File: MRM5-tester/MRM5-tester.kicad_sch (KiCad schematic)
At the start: 0 parts

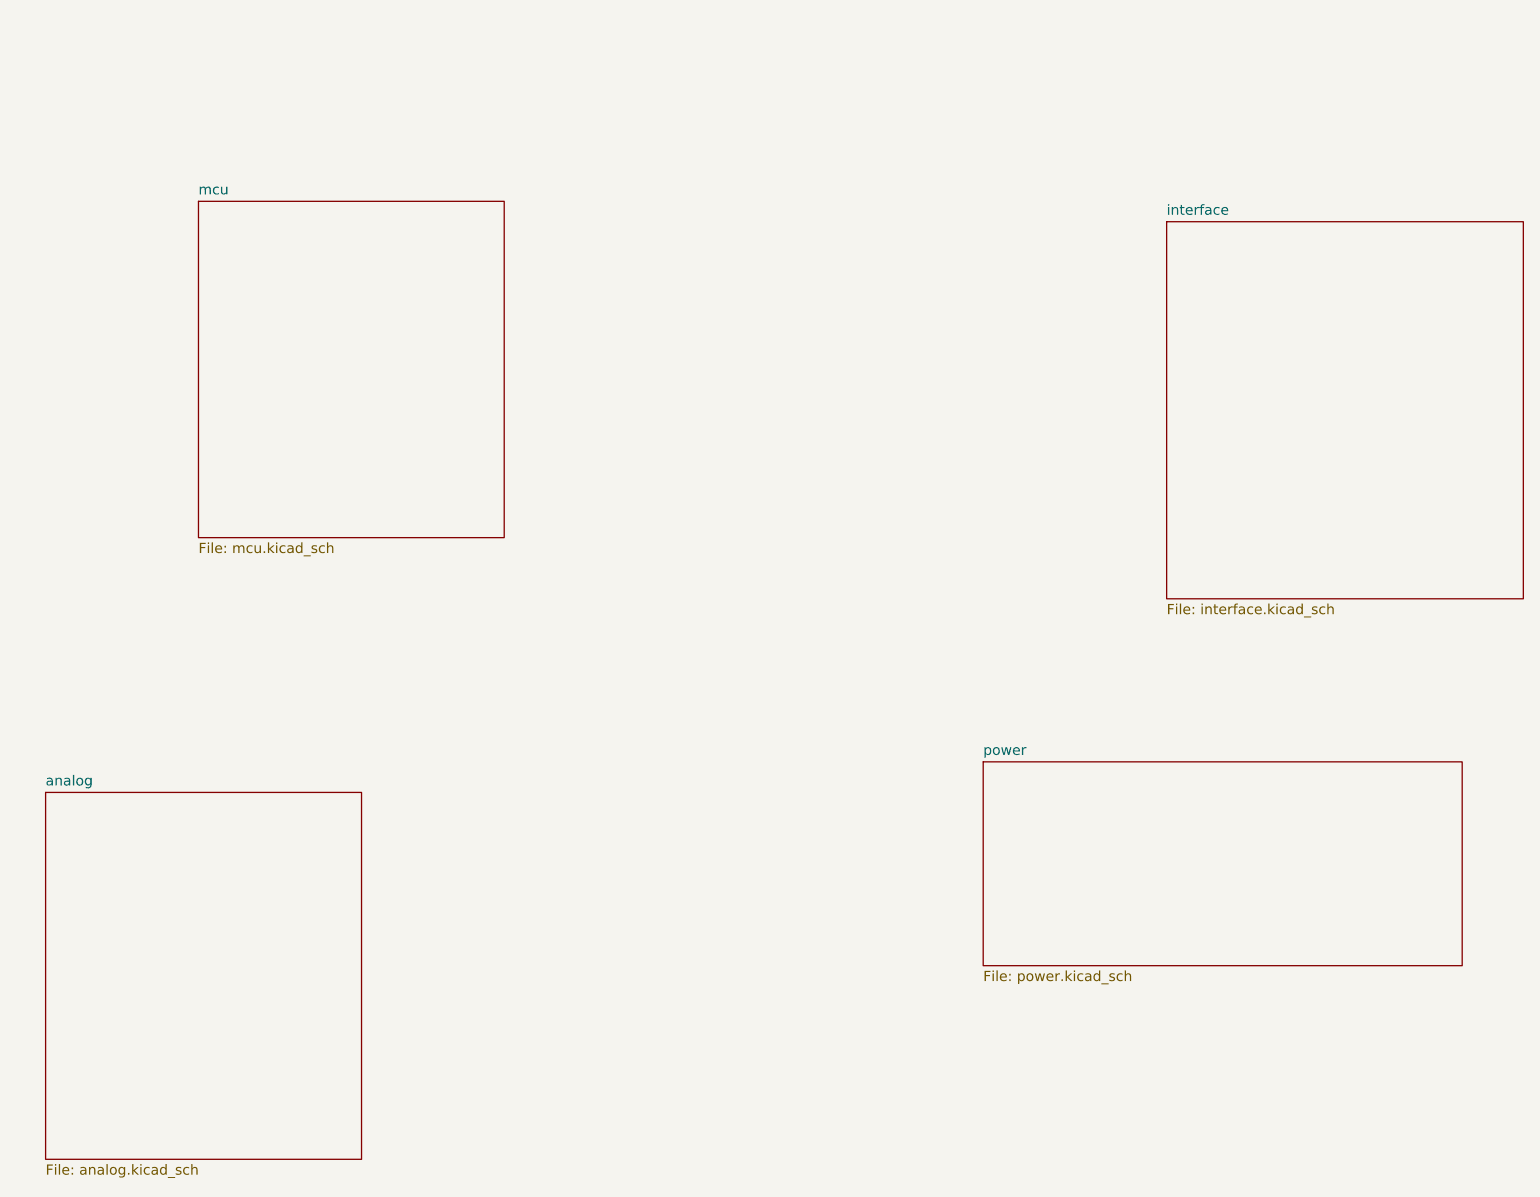
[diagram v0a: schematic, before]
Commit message: tester PCB 작성중
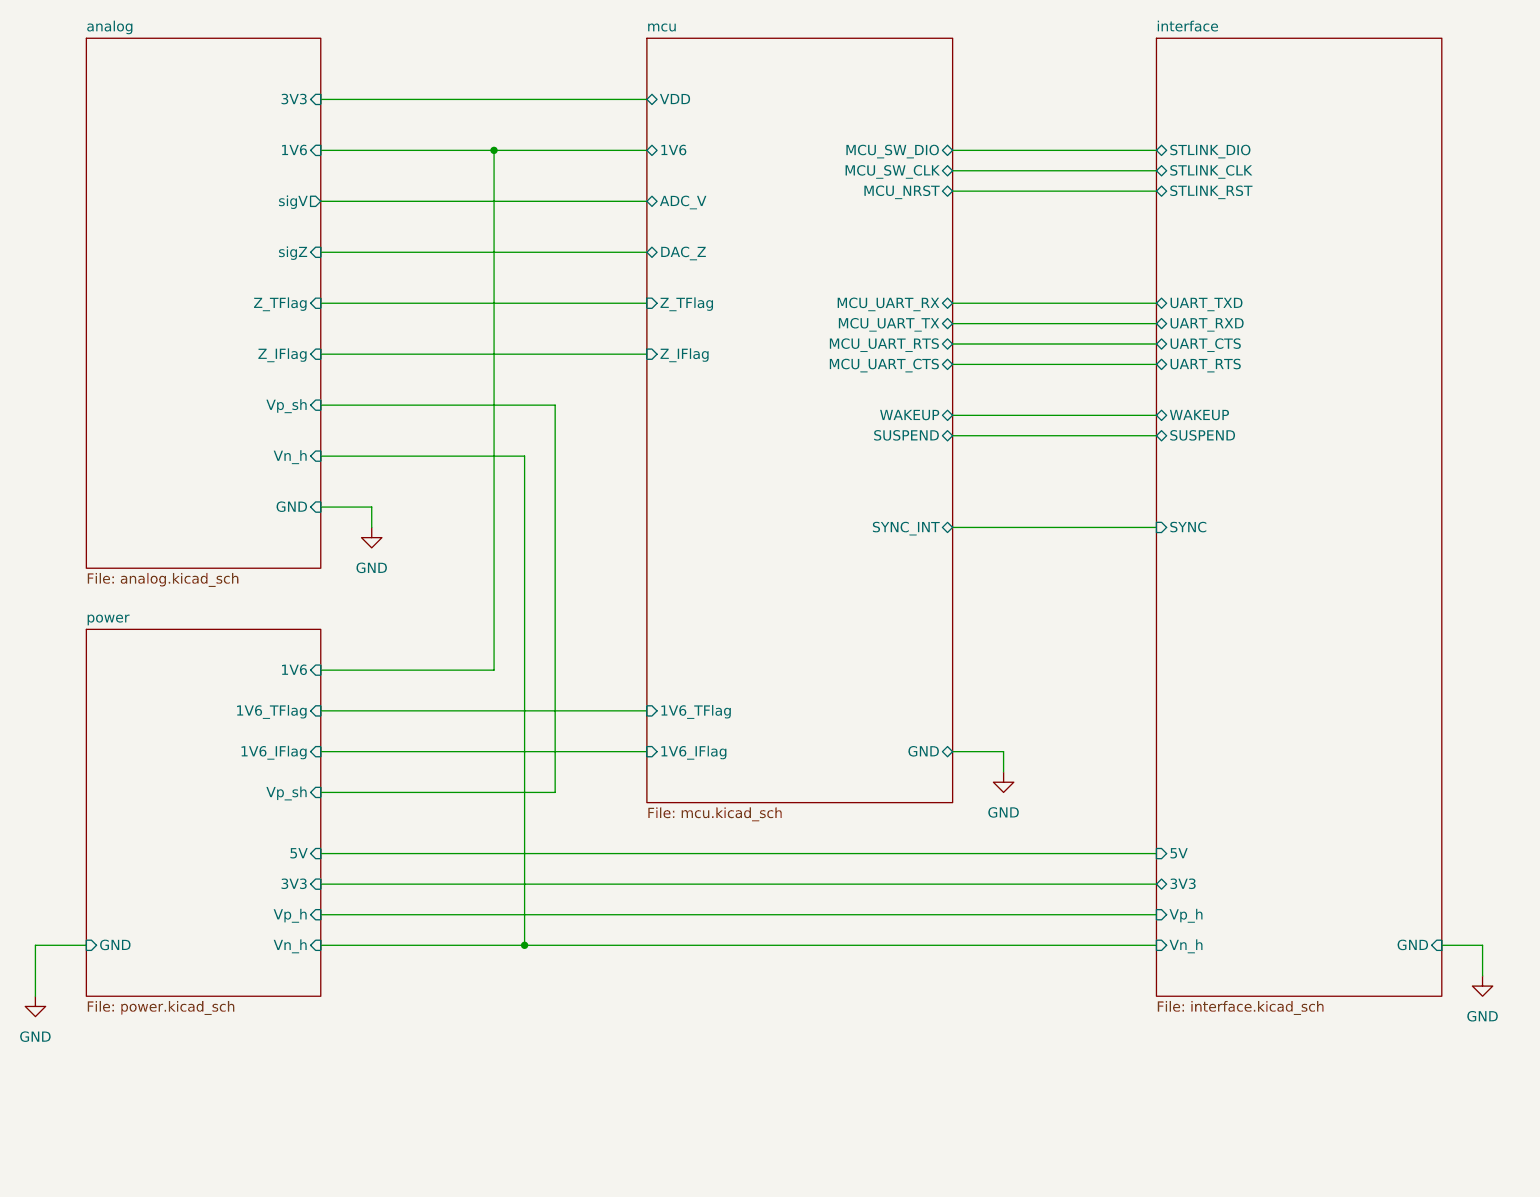
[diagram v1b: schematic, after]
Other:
- sheet analog ports: added 1V6, 3V3, GND, Vn_h, Vp_sh, Z_IFlag, Z_TFlag, sigV, sigZ; removed none
- sheet interface ports: added 3V3, 5V, GND, STLINK_CLK, STLINK_DIO, STLINK_RST, SUSPEND, SYNC, UART_CTS, UART_RTS, UART_RXD, UART_TXD, Vn_h, Vp_h, WAKEUP; removed none
- sheet mcu ports: added 1V6, 1V6_IFlag, 1V6_TFlag, ADC_V, DAC_Z, GND, MCU_NRST, MCU_SW_CLK, MCU_SW_DIO, MCU_UART_CTS, MCU_UART_RTS, MCU_UART_RX, MCU_UART_TX, SUSPEND, SYNC_INT, VDD, WAKEUP, Z_IFlag, Z_TFlag; removed none
- sheet power ports: added 1V6, 1V6_IFlag, 1V6_TFlag, 3V3, 5V, GND, Vn_h, Vp_h, Vp_sh; removed none
